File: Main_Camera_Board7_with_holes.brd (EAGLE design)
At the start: 127 x 44.2 mm, 8 parts

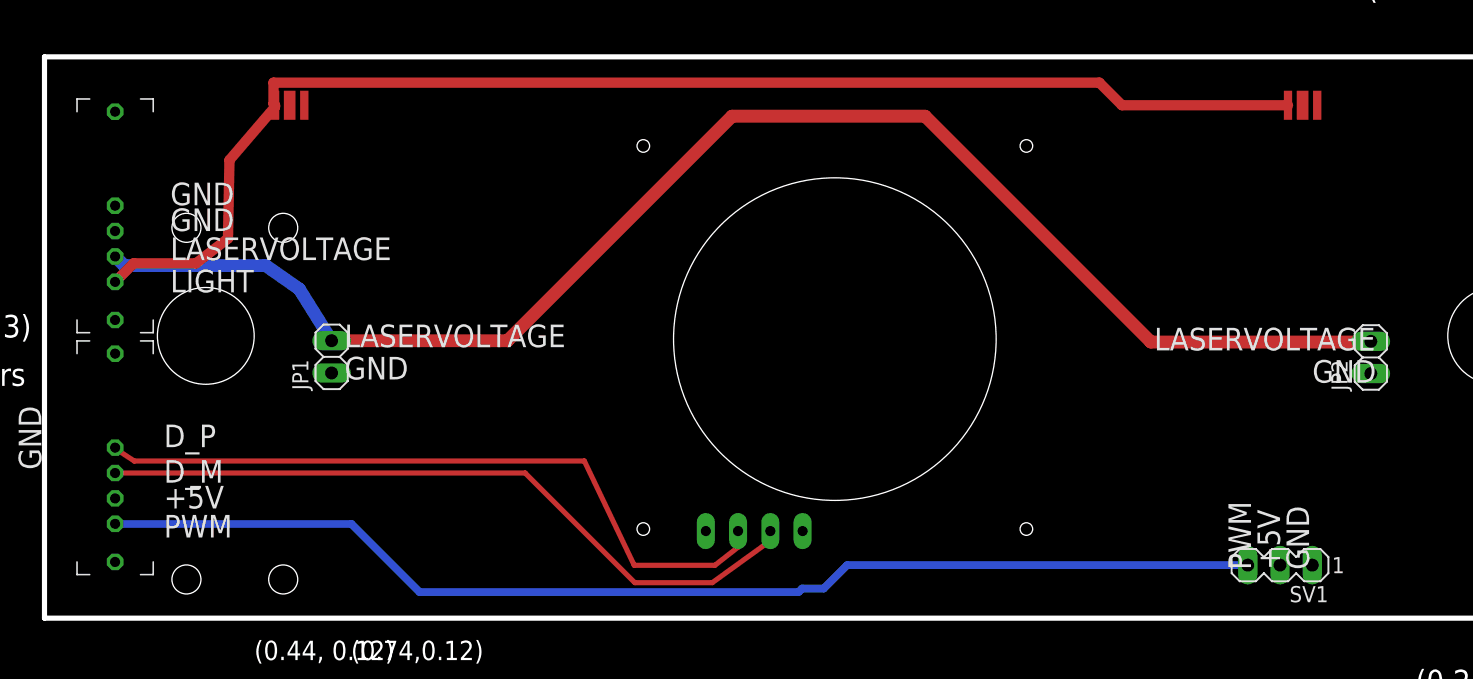
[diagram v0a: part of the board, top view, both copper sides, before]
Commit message: added luke made changes, moved connectors
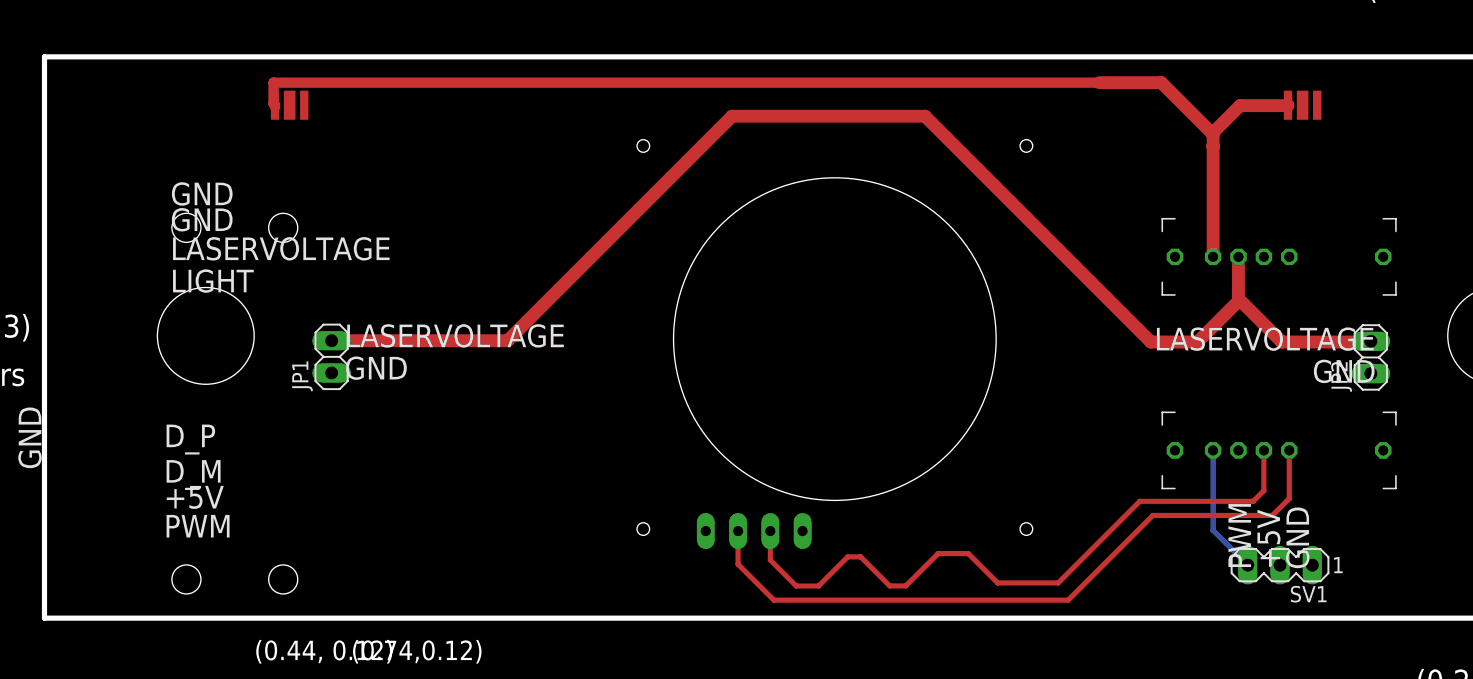
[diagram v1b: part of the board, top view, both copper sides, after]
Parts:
- moved U$4 100.5 mm to (101.6, 33.0), turned to 180 degrees
- moved U$5 100.1 mm to (101.6, 17.8), turned to 180 degrees
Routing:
- net PWM: track 92.3 -> 10.2 mm
- net LASER: track 116.7 -> 102.8 mm
- net LIGHT: track 104.4 -> 94.2 mm
- net D_M: track 57.0 -> 52.1 mm
- net D_P: track 56.4 -> 54.3 mm
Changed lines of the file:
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@@
 <setting verticaltext="up"/>
 </settings>
-<grid distance="0.0015625" unitdist="inch" unit="inch" style="lines" multiple="1" display="yes" altdistance="0.025" altunitdist="inch" altunit="inch"/>
+<grid distance="10" unitdist="mil" unit="mil" style="lines" multiple="1" display="yes" altdistance="0.025" altunitdist="inch" altunit="inch"/>
 <layers>
 <layer number="1" name="Top" color="4" fill="1" visible="yes" active="yes"/>
@@
 <element name="U$2" library="camera" package="LED" value="LED" x="15.494" y="44.958"/>
 <element name="U$3" library="camera" package="LED" value="LED" x="95.25" y="44.958"/>
-<element name="U$4" library="camera" package="T2I" value="T21" x="1.75" y="44.45" rot="R270"/>
-<element name="U$5" library="camera" package="T2I" value="T21" x="1.75" y="25.4" rot="R270"/>
+<element name="U$4" library="camera" package="T2I" value="T21" x="101.6" y="33.02" rot="R180"/>
+<element name="U$5" library="camera" package="T2I" value="T21" x="101.6" y="17.78" rot="R180"/>
 <element name="JP1" library="pinhead" package="1X02" value="" x="18.796" y="25.146" rot="R90"/>
 <element name="JP2" library="pinhead" package="1X02" value="" x="100.620375" y="25.099875" rot="R90"/>
@@
 <contactref element="U$1" pad="P$2"/>
 <contactref element="U$5" pad="P$3"/>
-<wire x1="53.34" y1="11.43" x2="53.34" y2="10.668" width="0.4064" layer="1"/>
-<wire x1="53.34" y1="10.668" x2="48.768" y2="7.366" width="0.4064" layer="1"/>
-<wire x1="1.75" y1="16" x2="34.038" y2="16" width="0.4064" layer="1"/>
-<wire x1="34.038" y1="16" x2="42.672" y2="7.366" width="0.4064" layer="1"/>
-<wire x1="42.672" y1="7.366" x2="48.768" y2="7.366" width="0.4064" layer="1"/>
+<wire x1="92.2" y1="17.78" x2="92.2" y2="14.6109375" width="0.4064" layer="1"/>
+<wire x1="92.2" y1="14.6109375" x2="91.360625" y2="13.7715625" width="0.4064" layer="1"/>
+<wire x1="91.360625" y1="13.7715625" x2="82.4309375" y2="13.7715625" width="0.4064" layer="1"/>
+<wire x1="82.4309375" y1="13.7715625" x2="76.0015625" y2="7.3421875" width="0.4064" layer="1"/>
+<wire x1="76.0015625" y1="7.3421875" x2="71.2390625" y2="7.3421875" width="0.4064" layer="1"/>
+<wire x1="55.3799375" y1="7.1040625" x2="53.34" y2="9.144" width="0.4064" layer="1"/>
+<wire x1="53.34" y1="9.144" x2="53.34" y2="11.43" width="0.4064" layer="1"/>
+<wire x1="55.3799375" y1="7.1040625" x2="57.1420625" y2="7.1040625" width="0.4064" layer="1"/>
+<wire x1="57.1420625" y1="7.1040625" x2="59.436" y2="9.398" width="0.4064" layer="1"/>
+<wire x1="59.436" y1="9.398" x2="60.452" y2="9.398" width="0.4064" layer="1"/>
+<wire x1="60.452" y1="9.398" x2="62.738" y2="7.112" width="0.4064" layer="1"/>
+<wire x1="62.738" y1="7.112" x2="64.008" y2="7.112" width="0.4064" layer="1"/>
+<wire x1="64.008" y1="7.112" x2="66.548" y2="9.652" width="0.4064" layer="1"/>
+<wire x1="66.548" y1="9.652" x2="68.92925" y2="9.652" width="0.4064" layer="1"/>
+<wire x1="68.92925" y1="9.652" x2="71.2390625" y2="7.3421875" width="0.4064" layer="1"/>
 </signal>
 <signal name="D_P">
 <contactref element="U$1" pad="P$3"/>
 <contactref element="U$5" pad="P$2"/>
-<wire x1="1.75" y1="18" x2="1.75" y2="17.935" width="0.4064" layer="1"/>
-<wire x1="1.75" y1="17.935" x2="3.254375" y2="16.9465625" width="0.4064" layer="1"/>
-<wire x1="3.254375" y1="16.9465625" x2="38.6953125" y2="16.9465625" width="0.4064" layer="1"/>
-<wire x1="38.6953125" y1="16.9465625" x2="42.624375" y2="8.73125" width="0.4064" layer="1"/>
-<wire x1="42.624375" y1="8.73125" x2="48.974375" y2="8.73125" width="0.4064" layer="1"/>
-<wire x1="48.974375" y1="8.73125" x2="50.8" y2="10.16" width="0.4064" layer="1"/>
-<wire x1="50.8" y1="10.16" x2="50.8" y2="11.43" width="0.4064" layer="1"/>
+<wire x1="94.2" y1="17.78" x2="94.2" y2="13.9915625" width="0.4064" layer="1"/>
+<wire x1="94.2" y1="13.9915625" x2="92.86875" y2="12.6603125" width="0.4064" layer="1"/>
+<wire x1="92.86875" y1="12.6603125" x2="83.4628125" y2="12.6603125" width="0.4064" layer="1"/>
+<wire x1="83.4628125" y1="12.6603125" x2="76.7953125" y2="5.9928125" width="0.4064" layer="1"/>
+<wire x1="76.7953125" y1="5.9928125" x2="53.6178125" y2="5.9928125" width="0.4064" layer="1"/>
+<wire x1="53.6178125" y1="5.9928125" x2="50.8" y2="8.810625" width="0.4064" layer="1"/>
+<wire x1="50.8" y1="8.810625" x2="50.8" y2="11.43" width="0.4064" layer="1"/>
 </signal>
 <signal name="N$2">
@@
 <contactref element="JP2" pad="2"/>
 <contactref element="U$4" pad="P$4"/>
-<wire x1="13.606625" y1="32.335625" x2="16.256" y2="30.48" width="1.016" layer="16"/>
-<wire x1="16.256" y1="30.48" x2="18.796" y2="26.416" width="1.016" layer="16"/>
-<wire x1="13.606625" y1="32.335625" x2="2.464375" y2="32.335625" width="1.016" layer="16"/>
-<wire x1="2.464375" y1="32.335625" x2="1.75" y2="33.05" width="1.016" layer="16"/>
 <wire x1="18.796" y1="26.416" x2="32.6469375" y2="26.416" width="1.016" layer="1"/>
 <wire x1="32.6469375" y1="26.416" x2="50.32375" y2="44.0928125" width="1.016" layer="1"/>
 <wire x1="50.32375" y1="44.0928125" x2="65.5240625" y2="44.0928125" width="1.016" layer="1"/>
 <wire x1="65.5240625" y1="44.0928125" x2="83.3040625" y2="26.3128125" width="1.016" layer="1"/>
-<wire x1="83.3040625" y1="26.3128125" x2="100.5633125" y2="26.3128125" width="1.016" layer="1"/>
 <wire x1="100.5633125" y1="26.3128125" x2="100.620375" y2="26.369875" width="1.016" layer="1"/>
+<wire x1="90.2" y1="33.02" x2="90.2" y2="29.7259375" width="1.016" layer="1"/>
+<wire x1="90.2" y1="29.7259375" x2="90.2" y2="29.5371875" width="1.016" layer="1"/>
+<wire x1="90.2" y1="29.5371875" x2="90.2096875" y2="29.5275" width="1.016" layer="1"/>
+<wire x1="90.2" y1="29.5371875" x2="86.975625" y2="26.3128125" width="1.016" layer="1"/>
+<wire x1="86.975625" y1="26.3128125" x2="83.3040625" y2="26.3128125" width="1.016" layer="1"/>
+<wire x1="100.5633125" y1="26.3128125" x2="93.613125" y2="26.3128125" width="1.016" layer="1"/>
+<wire x1="93.613125" y1="26.3128125" x2="90.2" y2="29.7259375" width="1.016" layer="1"/>
 </signal>
 <signal name="N$7">
@@
 <contactref element="SV1" pad="3"/>
 <contactref element="U$5" pad="P$5"/>
-<wire x1="90.932" y1="8.747125" x2="59.388375" y2="8.747125" width="0.6096" layer="16"/>
-<wire x1="59.388375" y1="8.747125" x2="57.546875" y2="6.905625" width="0.6096" layer="16"/>
-<wire x1="57.546875" y1="6.905625" x2="55.8403125" y2="6.905625" width="0.6096" layer="16"/>
-<wire x1="55.8403125" y1="6.905625" x2="55.5625" y2="6.6278125" width="0.6096" layer="16"/>
-<wire x1="55.5625" y1="6.6278125" x2="25.7175" y2="6.6278125" width="0.6096" layer="16"/>
-<wire x1="25.7175" y1="6.6278125" x2="20.3596875" y2="11.985625" width="0.6096" layer="16"/>
-<wire x1="20.3596875" y1="11.985625" x2="1.764375" y2="11.985625" width="0.6096" layer="16"/>
-<wire x1="1.764375" y1="11.985625" x2="1.75" y2="12" width="0.6096" layer="16"/>
+<wire x1="88.2" y1="17.78" x2="88.2" y2="11.479125" width="0.4064" layer="16"/>
+<wire x1="88.2" y1="11.479125" x2="90.932" y2="8.747125" width="0.4064" layer="16"/>
 </signal>
 <signal name="LIGHT">
@@
 <contactref element="U$3" pad="P$2"/>
 <contactref element="U$4" pad="P$5"/>
-<wire x1="94.1" y1="44.958" x2="81.026" y2="44.958" width="0.8128" layer="1"/>
-<wire x1="81.026" y1="44.958" x2="79.248" y2="46.736" width="0.8128" layer="1"/>
 <wire x1="79.248" y1="46.736" x2="14.224" y2="46.736" width="0.8128" layer="1"/>
 <wire x1="14.224" y1="46.736" x2="14.224" y2="45.078" width="0.8128" layer="1"/>
 <wire x1="14.224" y1="45.078" x2="14.344" y2="44.958" width="0.8128" layer="1"/>
 <wire x1="14.344" y1="44.958" x2="14.344" y2="44.824" width="0.8128" layer="1"/>
-<wire x1="14.344" y1="44.824" x2="10.7553125" y2="40.64" width="0.8128" layer="1"/>
-<wire x1="3.212" y1="32.512" x2="1.75" y2="31.05" width="0.8128" layer="1"/>
-<wire x1="3.212" y1="32.512" x2="8.128" y2="32.512" width="0.8128" layer="1"/>
-<wire x1="8.128" y1="32.512" x2="10.63625" y2="34.464625" width="0.8128" layer="1"/>
-<wire x1="10.63625" y1="34.464625" x2="10.7553125" y2="40.64" width="0.8128" layer="1"/>
+<wire x1="88.2" y1="33.02" x2="88.2" y2="41.6971875" width="1.016" layer="1"/>
+<wire x1="88.2" y1="41.6971875" x2="88.185625" y2="41.7115625" width="1.016" layer="1"/>
+<wire x1="88.2" y1="41.6971875" x2="88.2" y2="42.6640625" width="1.016" layer="1"/>
+<wire x1="88.2" y1="42.6640625" x2="88.2" y2="42.7975" width="1.016" layer="1"/>
+<wire x1="88.2" y1="42.7975" x2="90.32875" y2="44.92625" width="1.016" layer="1"/>
+<wire x1="90.32875" y1="44.92625" x2="94.06825" y2="44.92625" width="1.016" layer="1"/>
+<wire x1="94.06825" y1="44.92625" x2="94.1" y2="44.958" width="1.016" layer="1"/>
+<wire x1="84.1280625" y1="46.736" x2="88.2" y2="42.6640625" width="1.016" layer="1"/>
+<wire x1="79.248" y1="46.736" x2="84.1280625" y2="46.736" width="1.016" layer="1"/>
 </signal>
 </signals>
